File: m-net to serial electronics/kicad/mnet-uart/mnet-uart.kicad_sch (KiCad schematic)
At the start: 11 parts, among them U1 LM741, U2 LM741

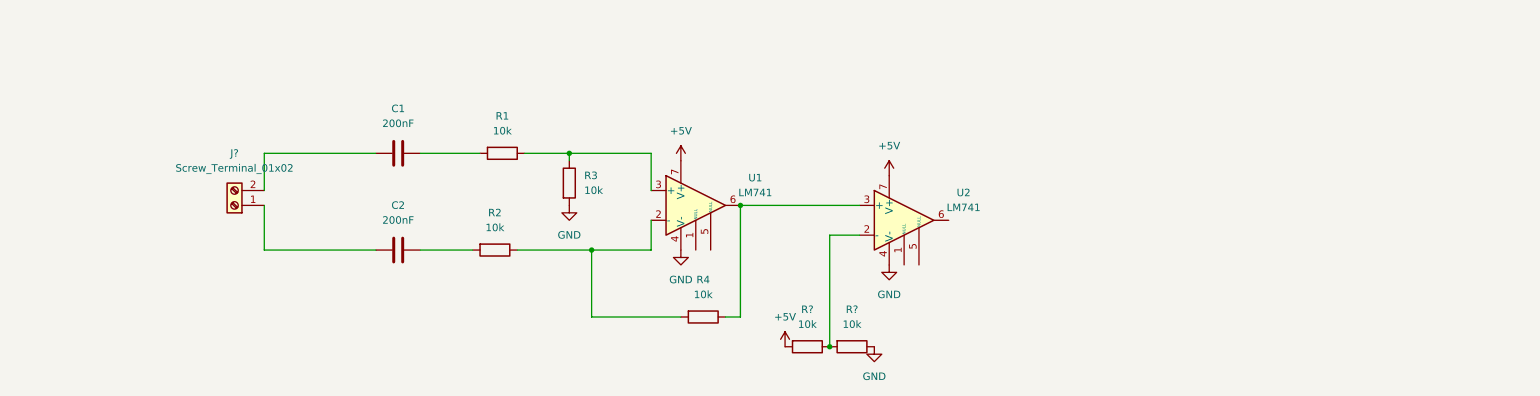
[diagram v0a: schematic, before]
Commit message: kicad schematics draft1
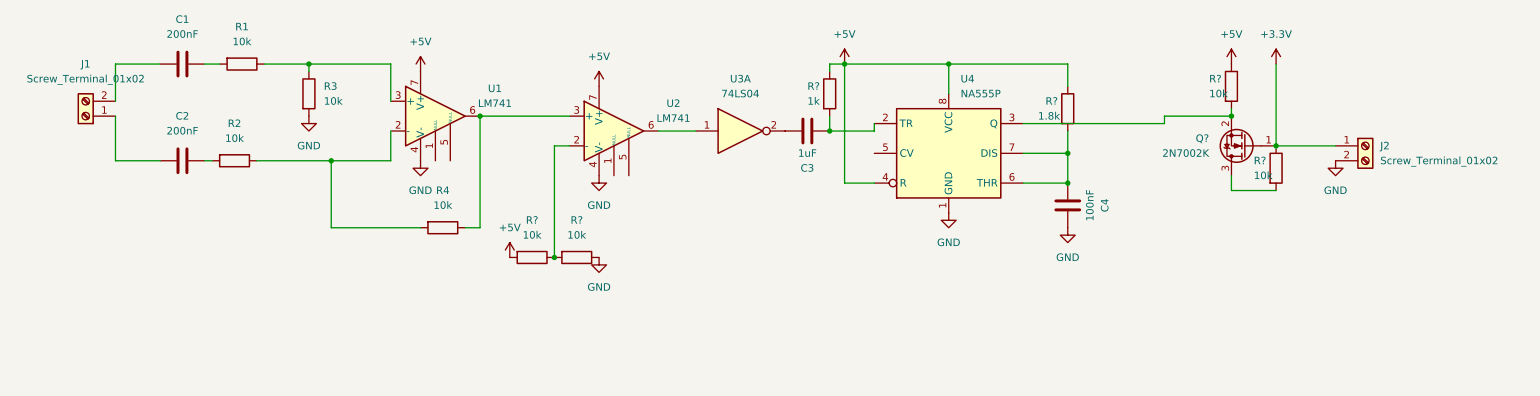
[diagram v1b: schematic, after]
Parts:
- added C3: 1uF, symbol Device:C
- added C4: 100nF, symbol Device:C
- added J2: Screw_Terminal_01x02, symbol Connector:Screw_Terminal_01x02
- added Q?: 2N7002K, Package_TO_SOT_SMD:SOT-23, symbol Transistor_FET:2N7002K
- added R?: 1.8k, symbol Device:R
- added R? (x2): 10k, symbol Device:R
- added R?: 1k, symbol Device:R
- added U3: 74LS04, symbol 74xx:74LS04
- added U4: NA555P, Package_DIP:DIP-8_W7.62mm, symbol Timer:NA555P
- gave numbers to parts that had none: 1
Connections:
- net +5V: now also R?.1, R?.1, R?.1, U4.4 (R), U4.8 (VCC)
- net GND: now also C4.1, J2.2 (Pin_2), U4.1 (GND)
- net at U2.6: now also U3.1
- new net: C3.1, U3.2
- new net: C3.2, R?.2, U4.2 (TR)
- new net: C4.2, R?.2, U4.6 (THR), U4.7 (DIS)
- new net: Q?.2 (S), R?.2, U4.3 (Q)
- new net: Q?.3 (D), R?.2
- new net +3.3V: J2.1 (Pin_1), Q?.1 (G), R?.1
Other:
- moved on the sheet: C1, C2, J1, R1, R2, R3, R4, R?, U1, U2
